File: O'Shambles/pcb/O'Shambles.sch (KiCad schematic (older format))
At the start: 128 parts, among them SW1 SW_PUSH, SW10 SW_PUSH, SW11 SW_PUSH, SW12 SW_PUSH, SW13 SW_PUSH, SW14 SW_PUSH, SW15 SW_PUSH, SW16 SW_PUSH, SW17 SW_PUSH, SW18 SW_PUSH, SW19 SW_PUSH, SW2 SW_PUSH, SW20 SW_PUSH, SW21 SW_PUSH, SW22 SW_PUSH, SW23 SW_PUSH, SW24 SW_PUSH, SW25 SW_PUSH, SW26 SW_PUSH, SW27 SW_PUSH, SW28 SW_PUSH, SW29 SW_PUSH, SW3 SW_PUSH, SW30 SW_PUSH, SW31 SW_PUSH, SW32 SW_PUSH, SW33 SW_PUSH, SW34 SW_PUSH, SW35 SW_PUSH, SW36 SW_PUSH, SW37 SW_PUSH, SW38 SW_PUSH, SW39 SW_PUSH, SW4 SW_PUSH, SW40 SW_PUSH, SW41 SW_PUSH, SW42 SW_PUSH, SW43 SW_PUSH, SW44 SW_PUSH, SW45 SW_PUSH, SW46 SW_PUSH, SW47 SW_PUSH, SW48 SW_PUSH, SW49 SW_PUSH, SW5 SW_PUSH, SW50 SW_PUSH, SW51 SW_PUSH, SW52 SW_PUSH, SW53 SW_PUSH, SW54 SW_PUSH, SW55 SW_PUSH, SW56 SW_PUSH, SW57 SW_PUSH, SW58 SW_PUSH, SW59 SW_PUSH, SW6 SW_PUSH, SW60 SW_PUSH, SW61 SW_PUSH, SW62 SW_PUSH, SW63 SW_PUSH, SW64 Rotary_Encoder_Switch, SW7 SW_PUSH, SW8 SW_PUSH, SW9 SW_PUSH, U1 ProMicro

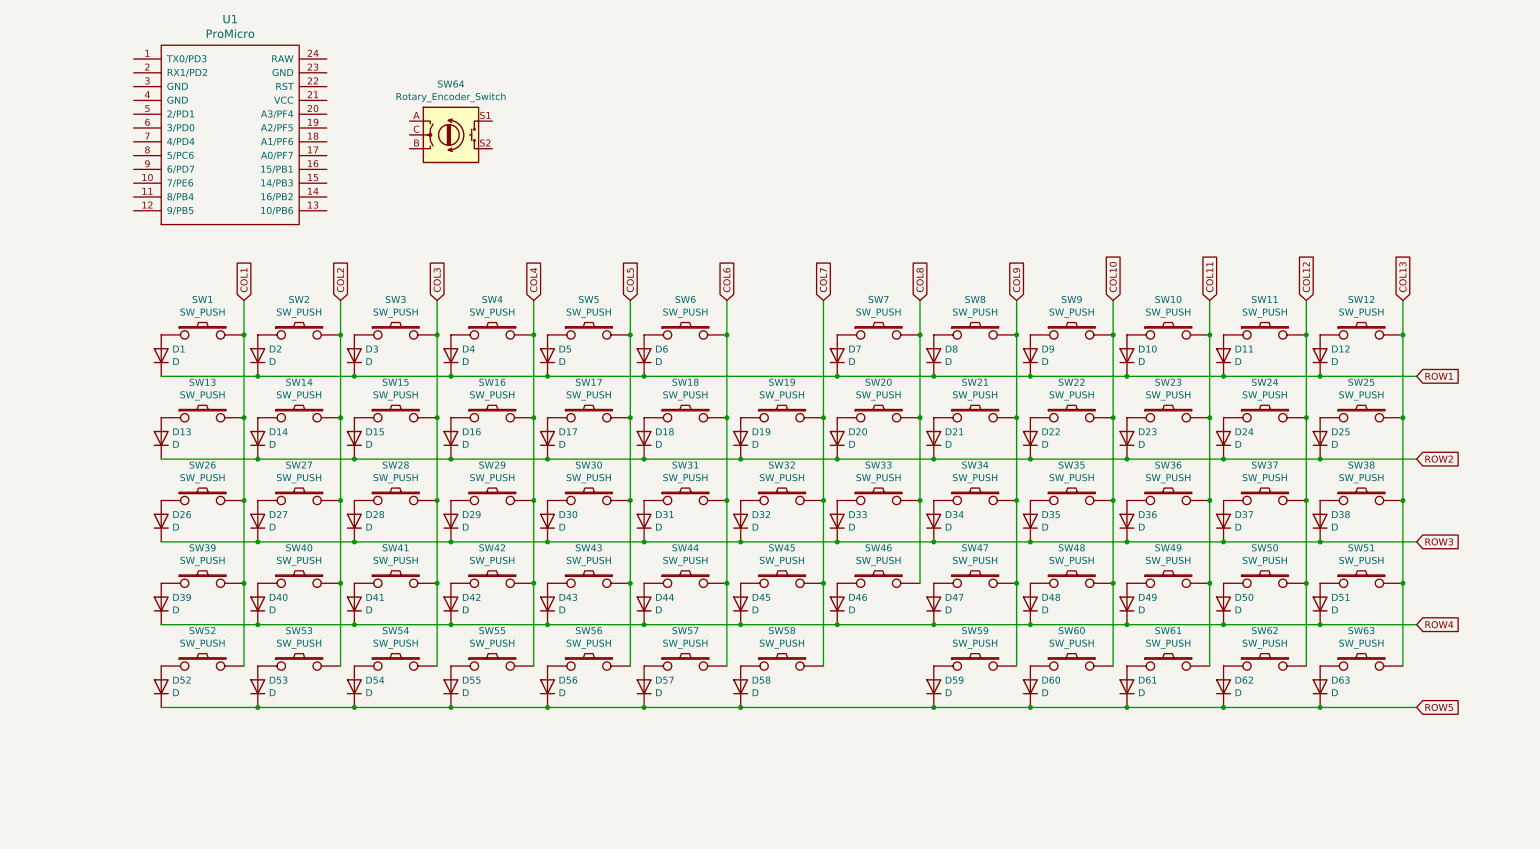
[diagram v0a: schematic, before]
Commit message: blockhead two, no ave, and some other boards
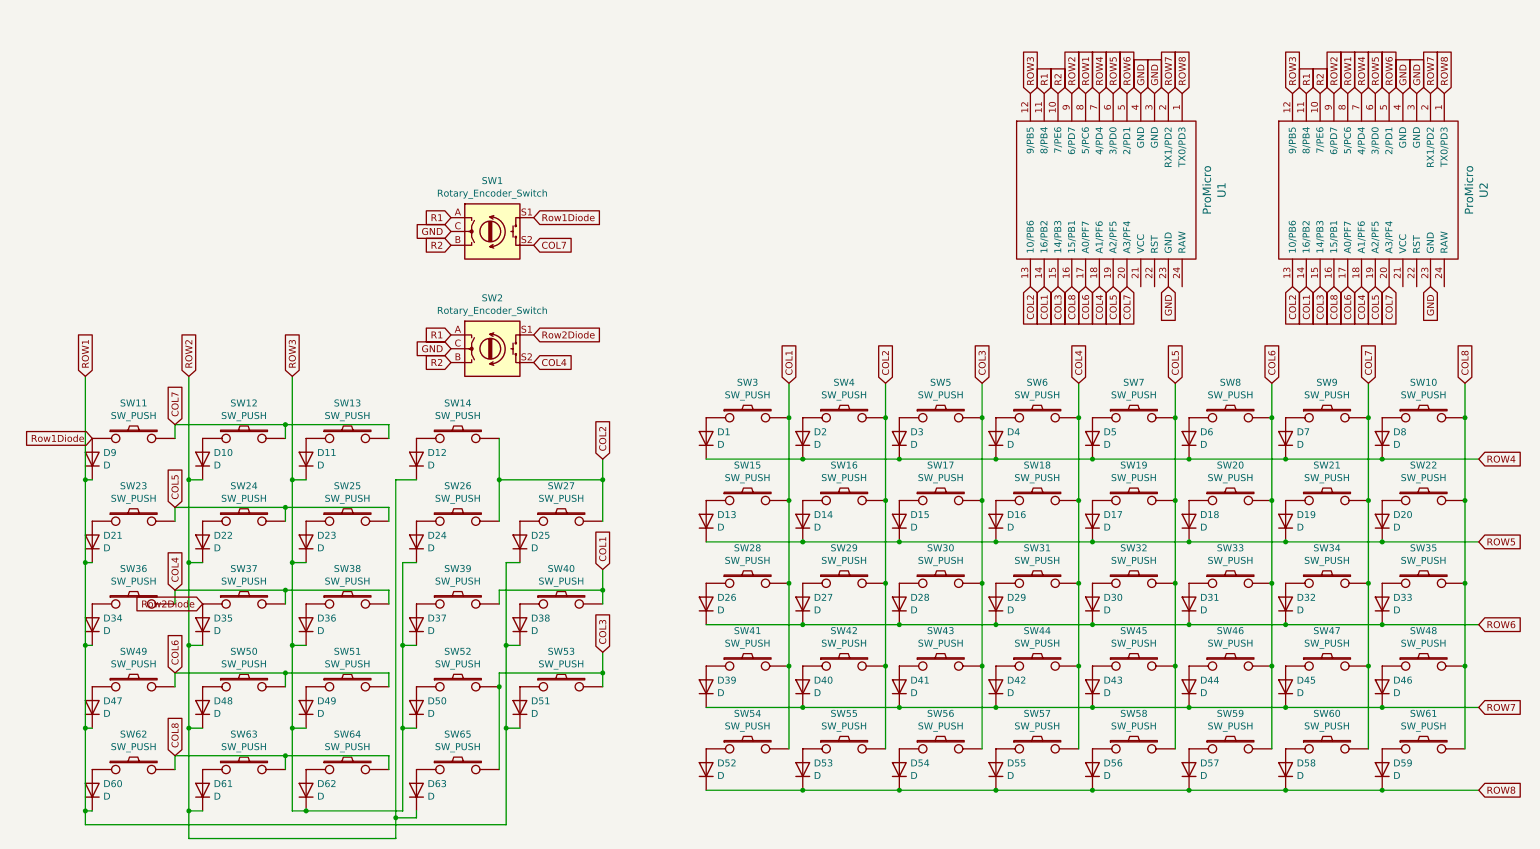
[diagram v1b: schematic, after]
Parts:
- added SW1: Rotary_Encoder_Switch, Keebio-Parts:RotaryEncoder_EC11, symbol Device:Rotary_Encoder_Switch
- added U1: ProMicro, Keebio-Parts:ArduinoProMicro, symbol keebio:ProMicro
- renumbered D5 to D1, D2 to D10, D3 to D11, D4 to D12, D18 to D13, D19 to D14, D20 to D15, D21 to D16, D22 to D17, D23 to D18, D24 to D19, D6 to D2, D25 to D20, D13 to D21, D14 to D22, D15 to D23, D16 to D24, D17 to D25, D31 to D26, D32 to D27, D33 to D28, D34 to D29, D7 to D3, D35 to D30, D36 to D31, D37 to D32, D38 to D33, D26 to D34, D27 to D35, D28 to D36, D29 to D37, D30 to D38, D44 to D39, D8 to D4, D45 to D40, D46 to D41, D47 to D42, D48 to D43, D49 to D44, D50 to D45, D51 to D46, D39 to D47, D40 to D48, D41 to D49, D9 to D5, D42 to D50, D43 to D51, D56 to D52, D57 to D53, D58 to D54, D59 to D55, D60 to D56, D61 to D57, D62 to D58, D63 to D59, D10 to D6, D52 to D60, D53 to D61, D54 to D62, D55 to D63, D11 to D7, D12 to D8, D1 to D9, SW12 to SW10, SW1 to SW11, SW2 to SW12, SW3 to SW13, SW4 to SW14, SW18 to SW15, SW19 to SW16, SW20 to SW17, SW21 to SW18, SW22 to SW19, SW64 to SW2, SW23 to SW20, SW24 to SW21, SW25 to SW22, SW13 to SW23, SW14 to SW24, SW15 to SW25, SW16 to SW26, SW17 to SW27, SW31 to SW28, SW32 to SW29, SW5 to SW3, SW33 to SW30, SW34 to SW31, SW35 to SW32, SW36 to SW33, SW37 to SW34, SW38 to SW35, SW26 to SW36, SW27 to SW37, SW28 to SW38, SW29 to SW39, SW6 to SW4, SW30 to SW40, SW44 to SW41, SW45 to SW42, SW46 to SW43, SW47 to SW44, SW48 to SW45, SW49 to SW46, SW50 to SW47, SW51 to SW48, SW39 to SW49, SW7 to SW5, SW40 to SW50, SW41 to SW51, SW42 to SW52, SW43 to SW53, SW56 to SW54, SW57 to SW55, SW58 to SW56, SW59 to SW57, SW60 to SW58, SW61 to SW59, SW8 to SW6, SW62 to SW60, SW63 to SW61, SW52 to SW62, SW53 to SW63, SW54 to SW64, SW55 to SW65, SW9 to SW7, SW10 to SW8, SW11 to SW9, U1 to U2
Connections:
- net COL10 is gone; now on net COL5: SW19.2, SW32.2, SW45.2, SW58.2, SW7.2
- net COL11 is gone; now on net COL6: SW20.2, SW33.2, SW46.2, SW59.2, SW8.2
- net COL12 is gone; now on net COL7: SW21.2, SW34.2, SW47.2, SW60.2, SW9.2
- net COL13 is gone; now on net COL8: SW10.2, SW22.2, SW35.2, SW48.2, SW61.2
- net COL9 is gone; now on net COL4: SW18.2, SW31.2, SW44.2, SW57.2, SW6.2
- net COL1: now also SW15.2, SW28.2, SW3.2, SW39.2, SW40.2, SW41.2, SW54.2, U2.14 (16/PB2), U1.14 (16/PB2); no longer SW11.2, SW23.2, SW36.2, SW49.2, SW62.2
- net COL2: now also SW14.2, SW16.2, SW26.2, SW27.2, SW29.2, SW4.2, SW42.2, SW55.2, U2.13 (10/PB6), U1.13 (10/PB6); no longer SW12.2, SW24.2, SW37.2, SW50.2, SW63.2
- net COL3: now also SW17.2, SW30.2, SW43.2, SW5.2, SW52.2, SW53.2, SW56.2, SW65.2, U2.15 (14/PB3), U1.15 (14/PB3); no longer SW13.2, SW25.2, SW38.2, SW51.2, SW64.2
- net COL4: now also SW2.S2, SW36.2, SW37.2, SW38.2, U2.18 (A1/PF6), U1.18 (A1/PF6); no longer SW14.2, SW26.2, SW39.2, SW52.2, SW65.2
- net COL5: now also SW23.2, SW24.2, SW25.2, U2.19 (A2/PF5), U1.19 (A2/PF5); no longer SW27.2, SW3.2, SW40.2, SW53.2, SW54.2
- net COL6: now also SW49.2, SW50.2, SW51.2, U2.17 (A0/PF7), U1.17 (A0/PF7); no longer SW15.2, SW28.2, SW4.2, SW41.2, SW55.2
- net COL7: now also SW11.2, SW12.2, SW13.2, U2.20 (A3/PF4), SW1.S2, U1.20 (A3/PF4); no longer SW16.2, SW29.2, SW42.2, SW56.2
- net COL8: now also SW62.2, SW63.2, SW64.2, U2.16 (15/PB1), U1.16 (15/PB1); no longer SW17.2, SW30.2, SW43.2, SW5.2
- net ROW1: now also D21.1 (K), D25.1 (K), D34.1 (K), D38.1 (K), D47.1 (K), D51.1 (K), D60.1 (K), U2.8 (5/PC6), U1.8 (5/PC6); no longer D1.1 (K), D10.1 (K), D11.1 (K), D12.1 (K), D2.1 (K), D3.1 (K), D4.1 (K), D5.1 (K), D6.1 (K), D7.1 (K), D8.1 (K)
- net ROW2: now also D10.1 (K), D12.1 (K), D35.1 (K), D48.1 (K), D61.1 (K), D63.1 (K), U2.9 (6/PD7), U1.9 (6/PD7); no longer D13.1 (K), D14.1 (K), D15.1 (K), D16.1 (K), D17.1 (K), D18.1 (K), D19.1 (K), D20.1 (K), D21.1 (K), D23.1 (K), D24.1 (K), D25.1 (K)
- net ROW3: now also D11.1 (K), D23.1 (K), D24.1 (K), D49.1 (K), D50.1 (K), D62.1 (K), U2.12 (9/PB5), U1.12 (9/PB5); no longer D26.1 (K), D27.1 (K), D28.1 (K), D29.1 (K), D30.1 (K), D31.1 (K), D32.1 (K), D33.1 (K), D34.1 (K), D35.1 (K), D38.1 (K)
- net ROW4: now also D1.1 (K), D2.1 (K), D3.1 (K), D4.1 (K), D5.1 (K), D6.1 (K), D7.1 (K), D8.1 (K), U2.7 (4/PD4), U1.7 (4/PD4); no longer D39.1 (K), D40.1 (K), D41.1 (K), D42.1 (K), D43.1 (K), D44.1 (K), D45.1 (K), D46.1 (K), D47.1 (K), D48.1 (K), D49.1 (K), D50.1 (K), D51.1 (K)
- net ROW5: now also D13.1 (K), D14.1 (K), D15.1 (K), D16.1 (K), D17.1 (K), D18.1 (K), D19.1 (K), D20.1 (K), U2.6 (3/PD0), U1.6 (3/PD0); no longer D52.1 (K), D53.1 (K), D54.1 (K), D55.1 (K), D56.1 (K), D57.1 (K), D58.1 (K), D59.1 (K), D60.1 (K), D61.1 (K), D62.1 (K), D63.1 (K)
- net Row1Diode: now reaches D9.2 (A), SW11.1
- net Row1Diode: now also SW1.S1
- net ROW8: now reaches U2.1 (TX0/PD3)
- net ROW8: now also D52.1 (K), D53.1 (K), D54.1 (K), D55.1 (K), D56.1 (K), D57.1 (K), D58.1 (K), D59.1 (K), U1.1 (TX0/PD3)
- net R2: now reaches U2.10 (7/PE6)
- net R2: now also SW2.B, SW1.B, U1.10 (7/PE6)
- net R1: now reaches U2.11 (8/PB4)
- net R1: now also SW2.A, SW1.A, U1.11 (8/PB4)
- net ROW7: now reaches U2.2 (RX1/PD2)
- net ROW7: now also D39.1 (K), D40.1 (K), D41.1 (K), D42.1 (K), D43.1 (K), D44.1 (K), D45.1 (K), D46.1 (K), U1.2 (RX1/PD2)
- net GND: now reaches U2.23 (GND)
- net GND: now also SW2.C, U2.3 (GND), U2.4 (GND), SW1.C, U1.23 (GND), U1.3 (GND), U1.4 (GND)
- net ROW6: now reaches U2.5 (2/PD1)
- net ROW6: now also D26.1 (K), D27.1 (K), D28.1 (K), D29.1 (K), D30.1 (K), D31.1 (K), D32.1 (K), D33.1 (K), U1.5 (2/PD1)
- net Row2Diode: now reaches D35.2 (A), SW37.1
- net Row2Diode: now also SW2.S1
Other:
- moved on the sheet: D1, D10, D11, D12, D13, D14, D15, D16, D17, D18, D19, D2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
